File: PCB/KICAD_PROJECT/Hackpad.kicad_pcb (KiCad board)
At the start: 2 copper layers, 62 x 89 mm, 21 parts, among them J1 OLED_128x64, SW1 RotaryEncoder_Switch, U1 MCU_Seeed_XIAO_RP2040

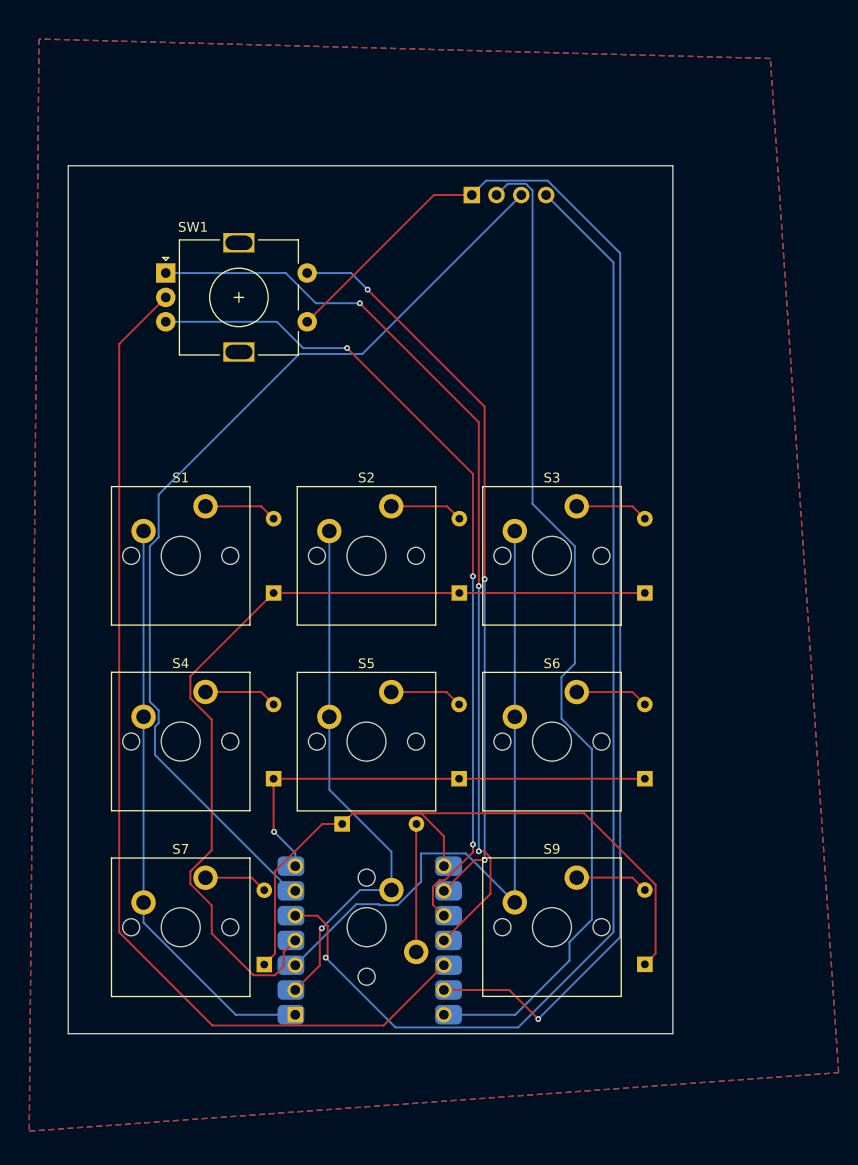
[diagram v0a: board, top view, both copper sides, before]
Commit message: sync
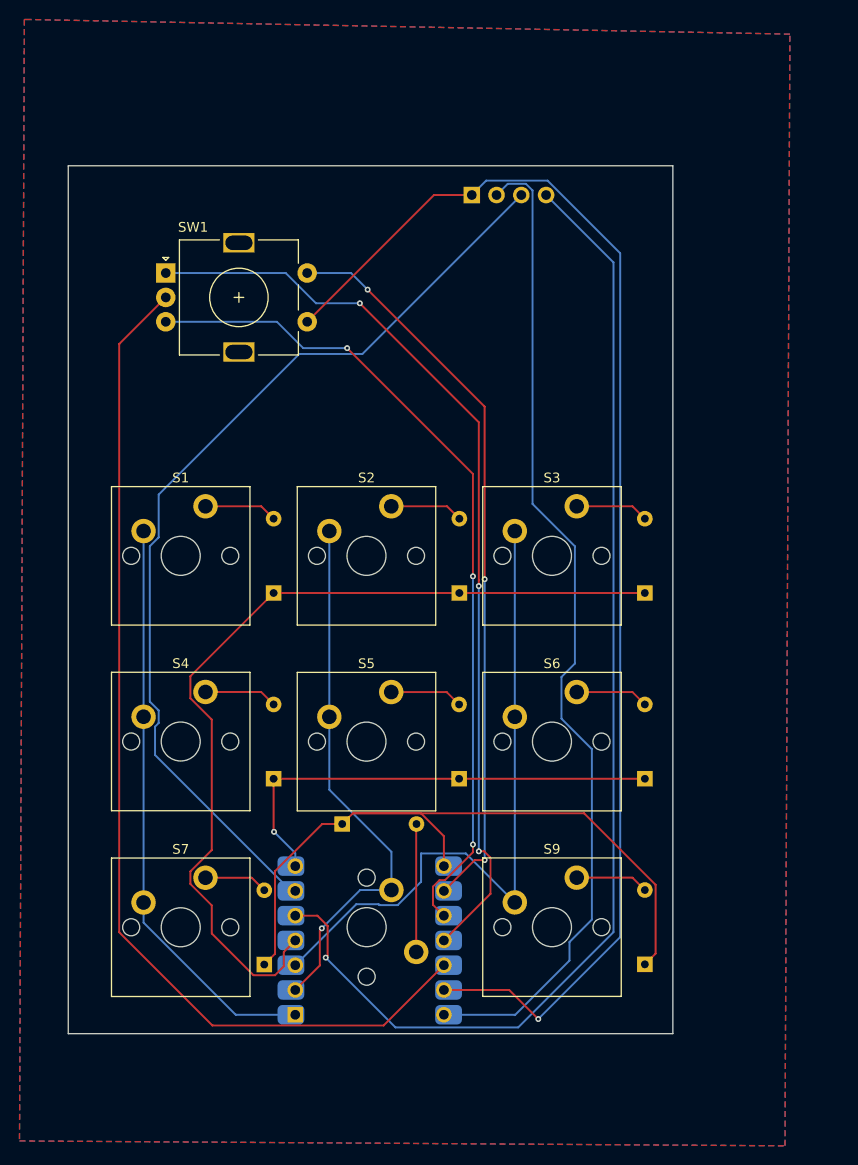
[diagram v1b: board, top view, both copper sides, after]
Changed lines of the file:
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@@
 		(polygon
 			(pts
-				(xy 35 59) (xy 34 171) (xy 117 165) (xy 110 61)
+				(xy 33.5 57) (xy 33 172) (xy 111.5 172.5) (xy 112 58.5) (xy 34 57)
 			)
 		)
